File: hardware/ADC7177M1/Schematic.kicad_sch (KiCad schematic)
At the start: 4 parts, among them J1 RFShield_OnePiece, J2 RFShield_OnePiece

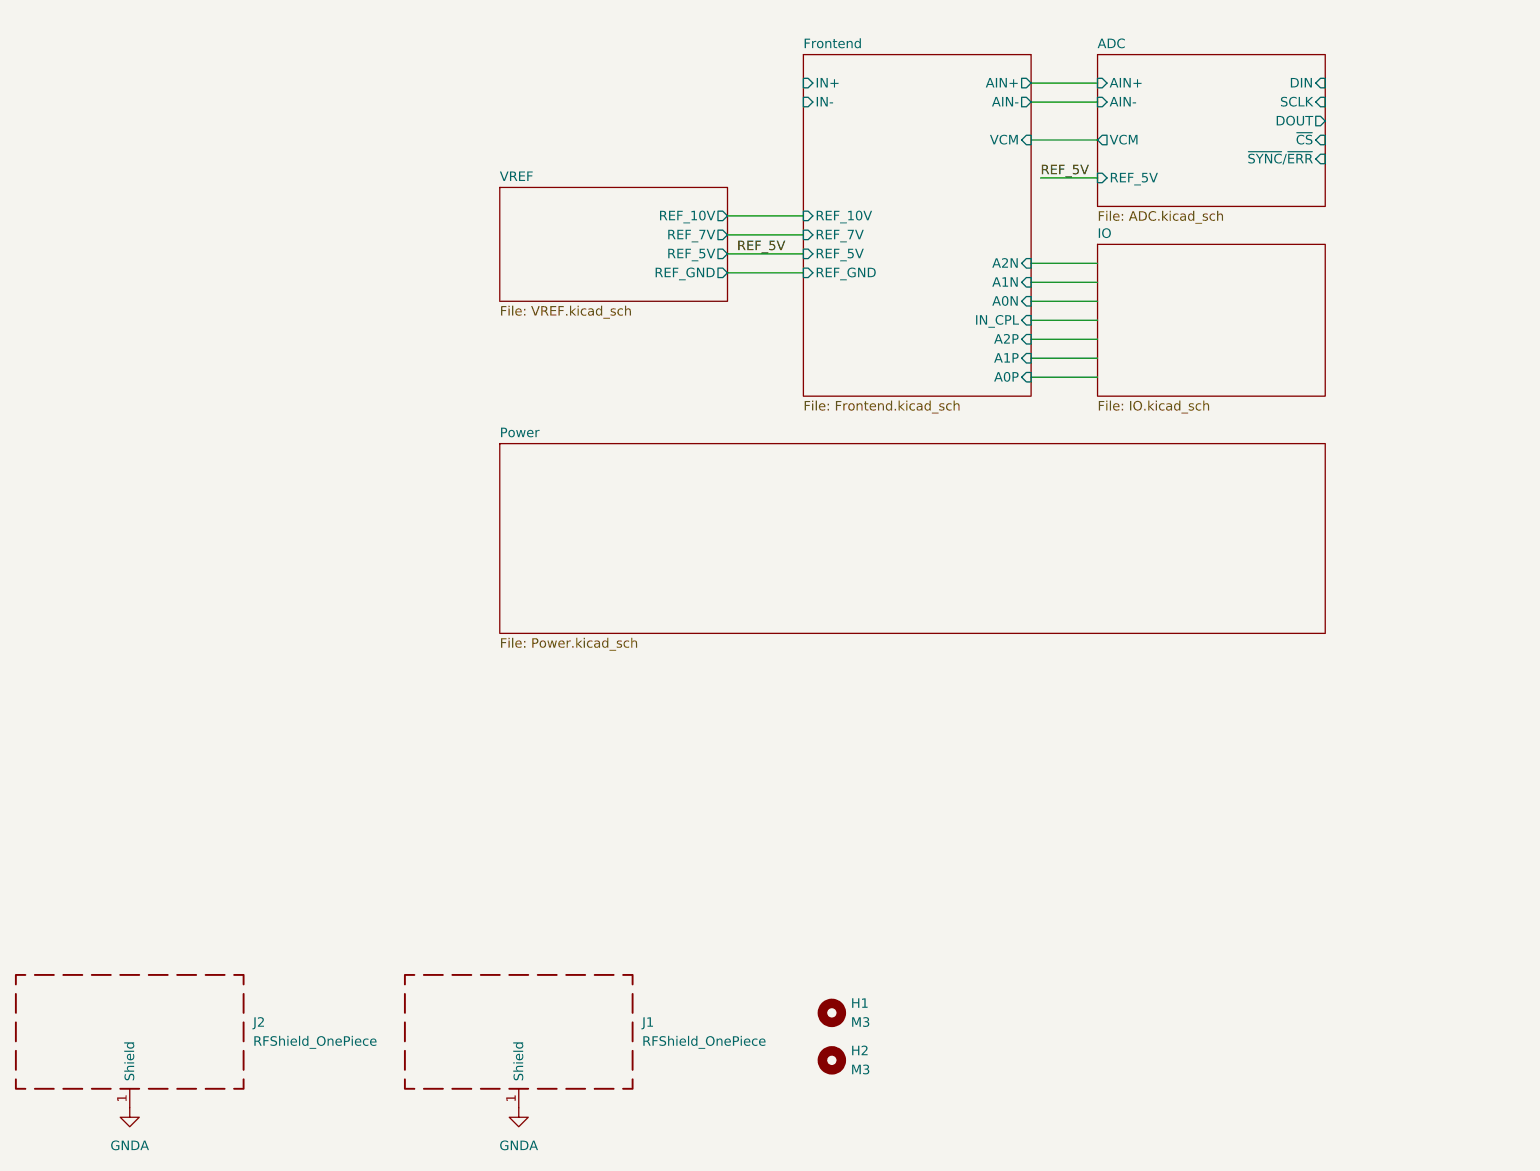
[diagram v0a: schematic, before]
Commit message: Schematic
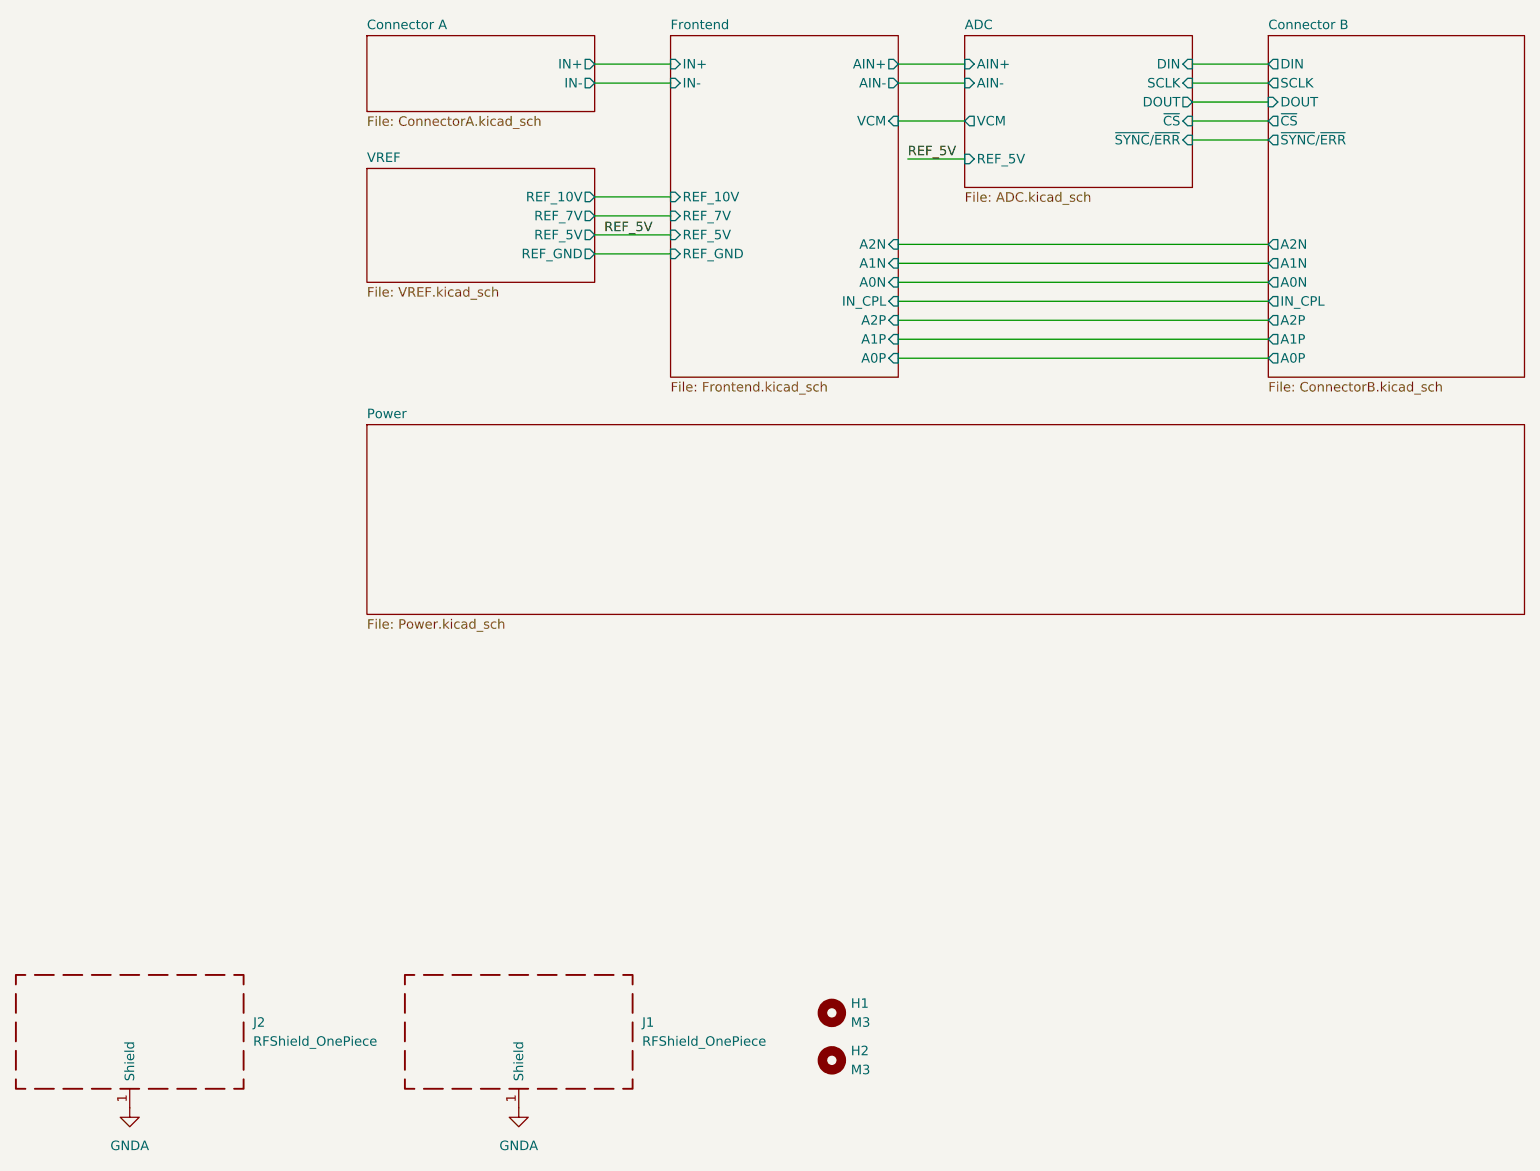
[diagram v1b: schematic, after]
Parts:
- H1, H2: footprint (none) -> MountingHole:MountingHole_3.2mm_M3_DIN965_Pad_TopBottom
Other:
- removed sheet IO
- added sheet Connector A (ConnectorA.kicad_sch)
- added sheet Connector B (ConnectorB.kicad_sch)
